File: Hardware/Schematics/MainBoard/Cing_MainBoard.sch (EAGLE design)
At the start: 179 parts, among them IC1 L293D, IC2 LM2576S, IC3 FT232RL, IC5 BME280, Q1 16mhz, Q2 BSS138, Q3 BSS138, Q4 BSS138, Q5 BSS138, Q6 NP2301AMR-G, Q7 NP2301AMR-G, U3 MPU-6050MPU6050

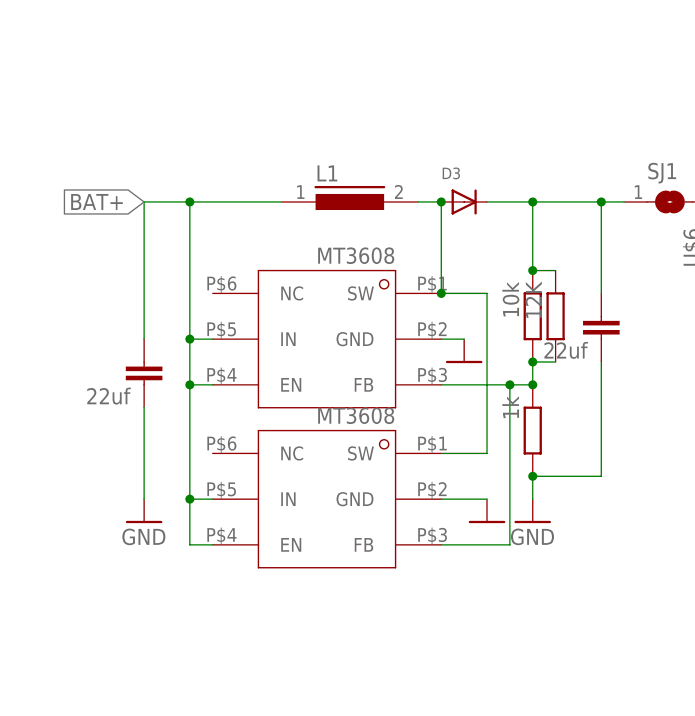
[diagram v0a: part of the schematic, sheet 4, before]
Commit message: commit
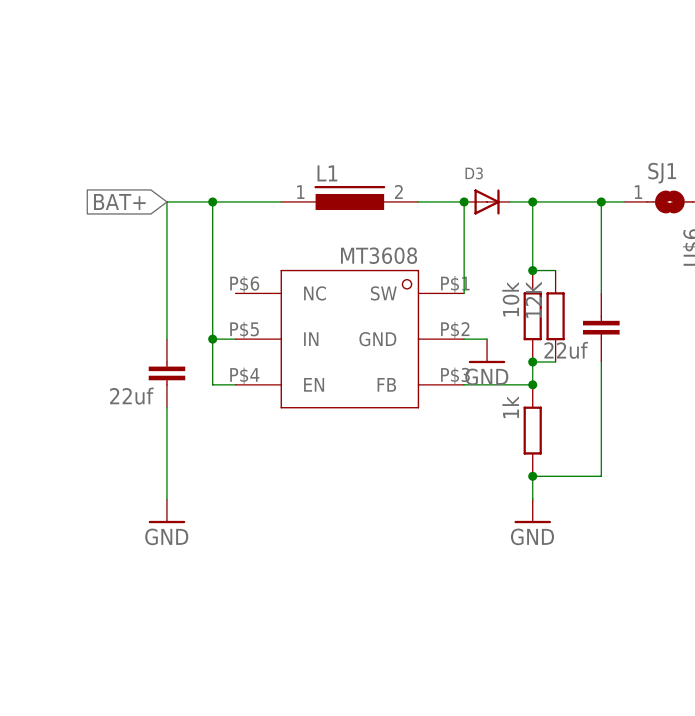
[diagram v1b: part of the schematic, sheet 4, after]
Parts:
- removed U$10: MT3608SOT23-6, MT3608:MT3608SOT23-6
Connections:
- removed net N$67: D3.A, L1.2, U$10.SW, U$5.SW
- new net N$44: D3.A, L1.2, U$5.SW
- net +3V3: now also IC1.VCC1
- net BAT+: no longer U$10.EN, U$10.IN
- net GND: no longer U$10.GND
- net N$35: no longer U$10.FB
- net VCC_SERVO: no longer IC1.VCC1
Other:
- moved on the sheet: D3

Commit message: commit
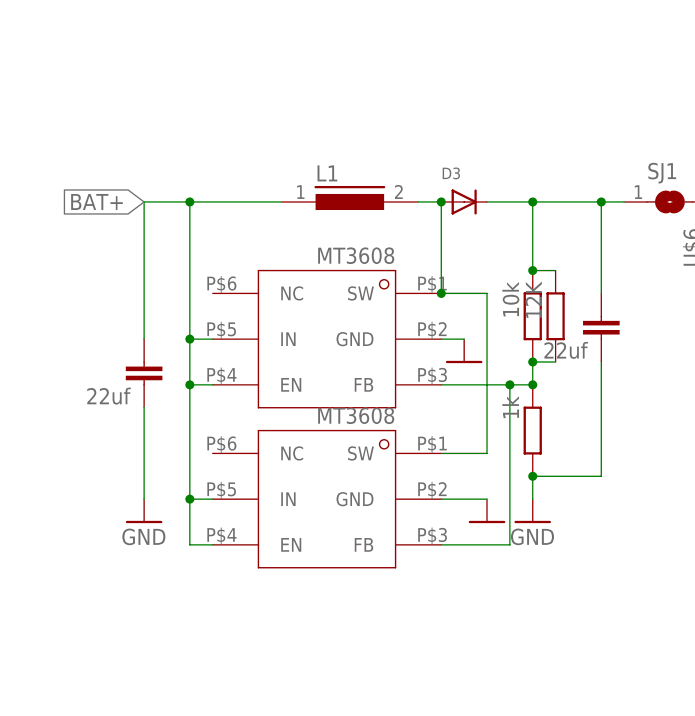
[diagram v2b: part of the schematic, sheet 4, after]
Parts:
- added U$10: MT3608SOT23-6, MT3608:MT3608SOT23-6
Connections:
- removed net N$44: D3.A, L1.2, U$5.SW
- new net N$67: D3.A, L1.2, U$10.SW, U$5.SW
- net BAT+: now also U$10.EN, U$10.IN
- net GND: now also U$10.GND
- net N$35: now also U$10.FB
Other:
- moved on the sheet: D3
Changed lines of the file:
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@@
 <part name="C25" library="rcl" library_urn="urn:adsk.eagle:library:334" deviceset="C-EU" device="C1206" package3d_urn="urn:adsk.eagle:package:23618/2" override_package3d_urn="urn:adsk.eagle:package:11833761/2" override_package_urn="urn:adsk.eagle:footprint:23125/1" value="100n"/>
 <part name="C26" library="rcl" library_urn="urn:adsk.eagle:library:334" deviceset="C-EU" device="C1206" package3d_urn="urn:adsk.eagle:package:23618/2" override_package3d_urn="urn:adsk.eagle:package:11833761/2" override_package_urn="urn:adsk.eagle:footprint:23125/1" value="100n"/>
+<part name="U$10" library="MT3608" deviceset="MT3608" device="SOT23-6" override_package3d_urn="urn:adsk.eagle:package:11833700/2" override_package_urn="urn:adsk.eagle:footprint:11833701/1" value="MT3608SOT23-6"/>
+<part name="GND65" library="supply1" library_urn="urn:adsk.eagle:library:371" deviceset="GND" device=""/>
 </parts>
 <sheets>
@@
 <attribute name="VALUE" x="178.562" y="86.36" size="1.778" layer="96" font="vector" rot="R270" align="top-center"/>
 </instance>
-<instance part="U$5" gate="G$1" x="5.08" y="25.4" smashed="yes" rot="MR0"/>
+<instance part="U$5" gate="G$1" x="2.54" y="25.4" smashed="yes" rot="MR0"/>
 <instance part="L1" gate="G$1" x="45.72" y="55.88" smashed="yes">
 <attribute name="NAME" x="41.91" y="58.166" size="1.778" layer="95"/>
 </instance>
-<instance part="D3" gate="G$1" x="60.96" y="55.88" smashed="yes">
-<attribute name="NAME" x="58.42" y="58.42" size="1.27" layer="95"/>
-<attribute name="VALUE" x="58.42" y="52.07" size="1.27" layer="96"/>
+<instance part="D3" gate="G$1" x="58.42" y="55.88" smashed="yes">
+<attribute name="NAME" x="55.88" y="58.42" size="1.27" layer="95"/>
+<attribute name="VALUE" x="55.88" y="52.07" size="1.27" layer="96"/>
 </instance>
 <instance part="R8" gate="G$1" x="157.48" y="88.9" smashed="yes" rot="R270">
@@
 <attribute name="VALUE" x="62.738" y="34.29" size="1.778" layer="96" rot="R270"/>
 </instance>
-<instance part="GND55" gate="1" x="60.96" y="38.1" smashed="yes">
-<attribute name="VALUE" x="58.42" y="35.56" size="1.778" layer="96"/>
-</instance>
+<instance part="GND55" gate="1" x="58.42" y="38.1" smashed="yes"/>
 <instance part="C14" gate="G$1" x="73.66" y="43.18" smashed="yes" rot="MR0">
 <attribute name="VALUE" x="72.136" y="38.481" size="1.778" layer="96" rot="MR0"/>
 </instance>
-<instance part="C15" gate="G$1" x="25.4" y="38.1" smashed="yes" rot="MR0">
-<attribute name="VALUE" x="23.876" y="33.401" size="1.778" layer="96" rot="MR0"/>
+<instance part="C15" gate="G$1" x="22.86" y="38.1" smashed="yes" rot="MR0">
+<attribute name="VALUE" x="21.336" y="33.401" size="1.778" layer="96" rot="MR0"/>
 </instance>
 <instance part="GND56" gate="1" x="66.04" y="20.32" smashed="yes">
 <attribute name="VALUE" x="63.5" y="17.78" size="1.778" layer="96"/>
 </instance>
-<instance part="GND57" gate="1" x="25.4" y="20.32" smashed="yes">
-<attribute name="VALUE" x="22.86" y="17.78" size="1.778" layer="96"/>
+<instance part="GND57" gate="1" x="22.86" y="20.32" smashed="yes">
+<attribute name="VALUE" x="20.32" y="17.78" size="1.778" layer="96"/>
 </instance>
 <instance part="U$8" gate="G$1" x="121.92" y="48.26" smashed="yes" rot="R90">
@@
 <attribute name="VALUE" x="30.48" y="96.52" size="1.778" layer="96"/>
 </instance>
+<instance part="U$10" gate="G$1" x="2.54" y="7.62" smashed="yes" rot="MR0"/>
+<instance part="GND65" gate="1" x="60.96" y="20.32" smashed="yes"/>
 </instances>
 <busses>
@@
 <segment>
 <pinref part="U$5" gate="G$1" pin="IN"/>
-<wire x1="33.02" y1="40.64" x2="30.48" y2="40.64" width="0.1524" layer="91"/>
-<wire x1="30.48" y1="40.64" x2="30.48" y2="35.56" width="0.1524" layer="91"/>
+<wire x1="30.48" y1="40.64" x2="27.94" y2="40.64" width="0.1524" layer="91"/>
+<wire x1="27.94" y1="40.64" x2="27.94" y2="35.56" width="0.1524" layer="91"/>
 <pinref part="U$5" gate="G$1" pin="EN"/>
-<wire x1="30.48" y1="35.56" x2="33.02" y2="35.56" width="0.1524" layer="91"/>
+<wire x1="27.94" y1="35.56" x2="30.48" y2="35.56" width="0.1524" layer="91"/>
 <pinref part="L1" gate="G$1" pin="1"/>
 <pinref part="C15" gate="G$1" pin="1"/>
-<wire x1="30.48" y1="55.88" x2="38.1" y2="55.88" width="0.1524" layer="91"/>
-<wire x1="30.48" y1="40.64" x2="30.48" y2="55.88" width="0.1524" layer="91"/>
-<junction x="30.48" y="40.64"/>
-<junction x="30.48" y="55.88"/>
-<wire x1="25.4" y1="40.64" x2="25.4" y2="55.88" width="0.1524" layer="91"/>
-<wire x1="25.4" y1="55.88" x2="30.48" y2="55.88" width="0.1524" layer="91"/>
-<label x="25.4" y="55.88" size="1.778" layer="95" rot="R180" xref="yes"/>
+<wire x1="27.94" y1="55.88" x2="38.1" y2="55.88" width="0.1524" layer="91"/>
+<wire x1="27.94" y1="40.64" x2="27.94" y2="55.88" width="0.1524" layer="91"/>
+<junction x="27.94" y="40.64"/>
+<junction x="27.94" y="55.88"/>
+<wire x1="22.86" y1="40.64" x2="22.86" y2="55.88" width="0.1524" layer="91"/>
+<wire x1="22.86" y1="55.88" x2="27.94" y2="55.88" width="0.1524" layer="91"/>
+<label x="22.86" y="55.88" size="1.778" layer="95" rot="R180" xref="yes"/>
+<wire x1="27.94" y1="35.56" x2="27.94" y2="22.86" width="0.1524" layer="91"/>
+<junction x="27.94" y="35.56"/>
+<pinref part="U$10" gate="G$1" pin="EN"/>
+<wire x1="27.94" y1="22.86" x2="27.94" y2="17.78" width="0.1524" layer="91"/>
+<wire x1="27.94" y1="17.78" x2="30.48" y2="17.78" width="0.1524" layer="91"/>
+<pinref part="U$10" gate="G$1" pin="IN"/>
+<wire x1="30.48" y1="22.86" x2="27.94" y2="22.86" width="0.1524" layer="91"/>
+<junction x="27.94" y="22.86"/>
 </segment>
 <segment>
@@
 <pinref part="C15" gate="G$1" pin="2"/>
 <pinref part="GND57" gate="1" pin="GND"/>
-<wire x1="25.4" y1="22.86" x2="25.4" y2="33.02" width="0.1524" layer="91"/>
+<wire x1="22.86" y1="22.86" x2="22.86" y2="33.02" width="0.1524" layer="91"/>
 </segment>
 <segment>
@@
 <pinref part="U$5" gate="G$1" pin="GND"/>
 <pinref part="GND55" gate="1" pin="GND"/>
-<wire x1="60.96" y1="40.64" x2="58.42" y2="40.64" width="0.1524" layer="91"/>
+<wire x1="58.42" y1="40.64" x2="55.88" y2="40.64" width="0.1524" layer="91"/>
 </segment>
 <segment>
@@
 <pinref part="GND64" gate="1" pin="GND"/>
 <wire x1="33.02" y1="101.6" x2="33.02" y2="106.68" width="0.1524" layer="91"/>
+</segment>
+<segment>
+<pinref part="U$10" gate="G$1" pin="GND"/>
+<pinref part="GND65" gate="1" pin="GND"/>
+<wire x1="60.96" y1="22.86" x2="55.88" y2="22.86" width="0.1524" layer="91"/>
 </segment>
 </net>
@@
 <wire x1="66.04" y1="38.1" x2="66.04" y2="35.56" width="0.1524" layer="91"/>
 <pinref part="U$5" gate="G$1" pin="FB"/>
-<wire x1="58.42" y1="35.56" x2="66.04" y2="35.56" width="0.1524" layer="91"/>
+<wire x1="55.88" y1="35.56" x2="63.5" y2="35.56" width="0.1524" layer="91"/>
 <junction x="66.04" y="35.56"/>
 <pinref part="R49" gate="G$1" pin="2"/>
+<wire x1="63.5" y1="35.56" x2="66.04" y2="35.56" width="0.1524" layer="91"/>
 <wire x1="66.04" y1="38.1" x2="68.58" y2="38.1" width="0.1524" layer="91"/>
 <junction x="66.04" y="38.1"/>
-</segment>
-</net>
-<net name="N$44" class="0">
-<segment>
-<pinref part="L1" gate="G$1" pin="2"/>
-<pinref part="D3" gate="G$1" pin="A"/>
-<wire x1="58.42" y1="55.88" x2="53.34" y2="55.88" width="0.1524" layer="91"/>
-<pinref part="U$5" gate="G$1" pin="SW"/>
-<wire x1="58.42" y1="45.72" x2="58.42" y2="55.88" width="0.1524" layer="91"/>
-<junction x="58.42" y="55.88"/>
+<pinref part="U$10" gate="G$1" pin="FB"/>
+<wire x1="63.5" y1="35.56" x2="63.5" y2="17.78" width="0.1524" layer="91"/>
+<wire x1="63.5" y1="17.78" x2="55.88" y2="17.78" width="0.1524" layer="91"/>
+<junction x="63.5" y="35.56"/>
 </segment>
 </net>
@@
 <pinref part="D3" gate="G$1" pin="C"/>
 <pinref part="R9" gate="G$1" pin="1"/>
-<wire x1="63.5" y1="55.88" x2="66.04" y2="55.88" width="0.1524" layer="91"/>
+<wire x1="60.96" y1="55.88" x2="66.04" y2="55.88" width="0.1524" layer="91"/>
 <wire x1="66.04" y1="55.88" x2="66.04" y2="48.26" width="0.1524" layer="91"/>
 <wire x1="66.04" y1="55.88" x2="73.66" y2="55.88" width="0.1524" layer="91"/>
@@
 </segment>
 </net>
+<net name="N$67" class="0">
+<segment>
+<pinref part="U$10" gate="G$1" pin="SW"/>
+<wire x1="55.88" y1="27.94" x2="60.96" y2="27.94" width="0.1524" layer="91"/>
+<pinref part="L1" gate="G$1" pin="2"/>
+<pinref part="D3" gate="G$1" pin="A"/>
+<wire x1="55.88" y1="55.88" x2="53.34" y2="55.88" width="0.1524" layer="91"/>
+<pinref part="U$5" gate="G$1" pin="SW"/>
+<wire x1="55.88" y1="45.72" x2="55.88" y2="55.88" width="0.1524" layer="91"/>
+<junction x="55.88" y="55.88"/>
+<wire x1="60.96" y1="27.94" x2="60.96" y2="45.72" width="0.1524" layer="91"/>
+<wire x1="60.96" y1="45.72" x2="55.88" y2="45.72" width="0.1524" layer="91"/>
+<junction x="55.88" y="45.72"/>
+</segment>
+</net>

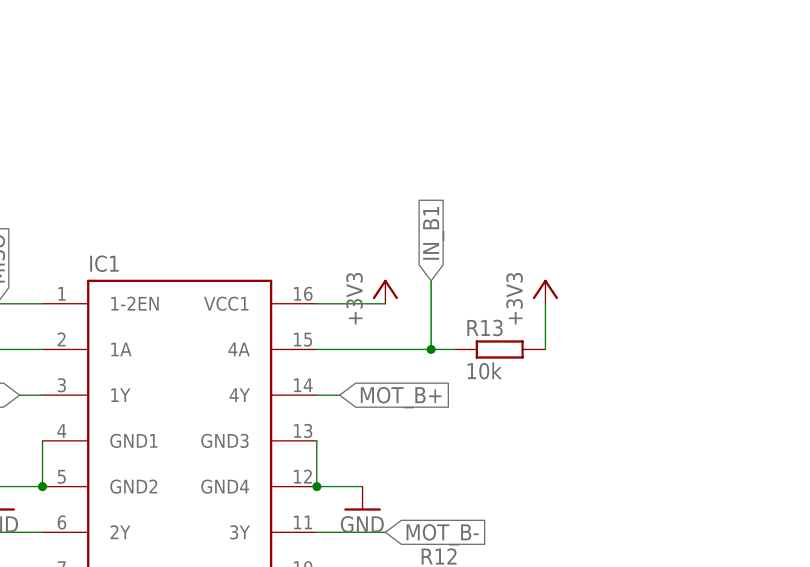
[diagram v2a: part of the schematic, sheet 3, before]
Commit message: commit
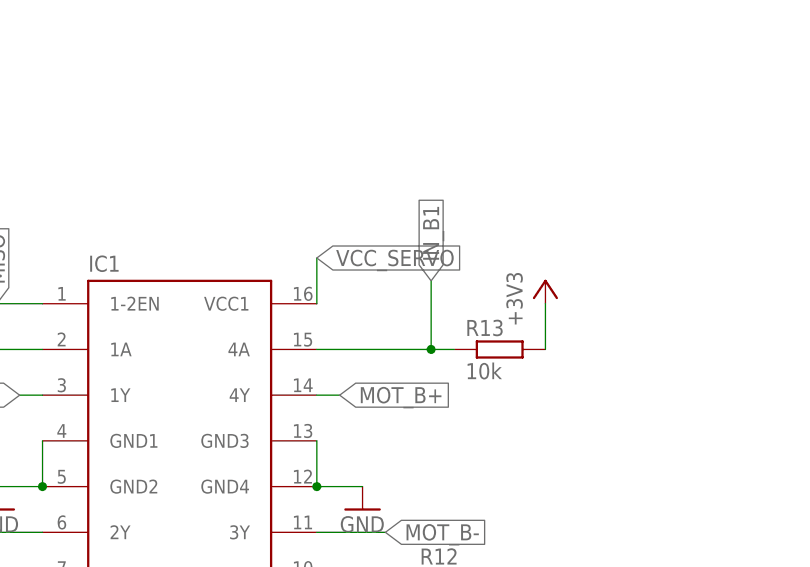
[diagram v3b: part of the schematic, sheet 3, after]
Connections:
- net +3V3: no longer IC1.VCC1
- net VCC_SERVO: now also IC1.VCC1
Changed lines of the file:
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@@
 <part name="+3V10" library="supply1" library_urn="urn:adsk.eagle:library:371" deviceset="+3V3" device=""/>
 <part name="+3V11" library="supply1" library_urn="urn:adsk.eagle:library:371" deviceset="+3V3" device=""/>
-<part name="+3V12" library="supply1" library_urn="urn:adsk.eagle:library:371" deviceset="+3V3" device=""/>
 <part name="R26" library="rcl" library_urn="urn:adsk.eagle:library:334" deviceset="R-EU_" device="R1206" package3d_urn="urn:adsk.eagle:package:23540/2" override_package3d_urn="urn:adsk.eagle:package:11835322/2" override_package_urn="urn:adsk.eagle:footprint:23047/1" value="40"/>
 <part name="GND35" library="supply1" library_urn="urn:adsk.eagle:library:371" deviceset="GND" device=""/>
@@
 <attribute name="VALUE" x="187.96" y="101.6" size="1.778" layer="96" rot="R90"/>
 </instance>
-<instance part="+3V12" gate="G$1" x="172.72" y="106.68" smashed="yes">
-<attribute name="VALUE" x="170.18" y="101.6" size="1.778" layer="96" rot="R90"/>
-</instance>
 <instance part="IC1" gate="G$1" x="149.86" y="86.36" smashed="yes">
 <attribute name="NAME" x="139.7" y="107.696" size="1.778" layer="95"/>
@@
 <pinref part="+3V11" gate="G$1" pin="+3V3"/>
 </segment>
-<segment>
-<wire x1="172.72" y1="104.14" x2="165.1" y2="104.14" width="0.1524" layer="91"/>
-<pinref part="+3V12" gate="G$1" pin="+3V3"/>
-<pinref part="IC1" gate="G$1" pin="VCC1"/>
-</segment>
 </net>
 <net name="D6" class="0">
@@
 <label x="33.02" y="144.78" size="1.778" layer="95" rot="R180" xref="yes"/>
 </segment>
-</net>
+<segment>
+<wire x1="165.1" y1="109.22" x2="165.1" y2="104.14" width="0.1524" layer="91"/>
+<label x="165.1" y="109.22" size="1.778" layer="95" xref="yes"/>
+<pinref part="IC1" gate="G$1" pin="VCC1"/>
+</segment>
+</net>
